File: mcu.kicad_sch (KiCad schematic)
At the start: 34 parts, among them J201 WIFI_ANT, J202 UART, SW201 BOOT_SEL, SW202 RST_SW, U201 ESP32C3, U202 W25Q32JVSS, Y202 40MHz

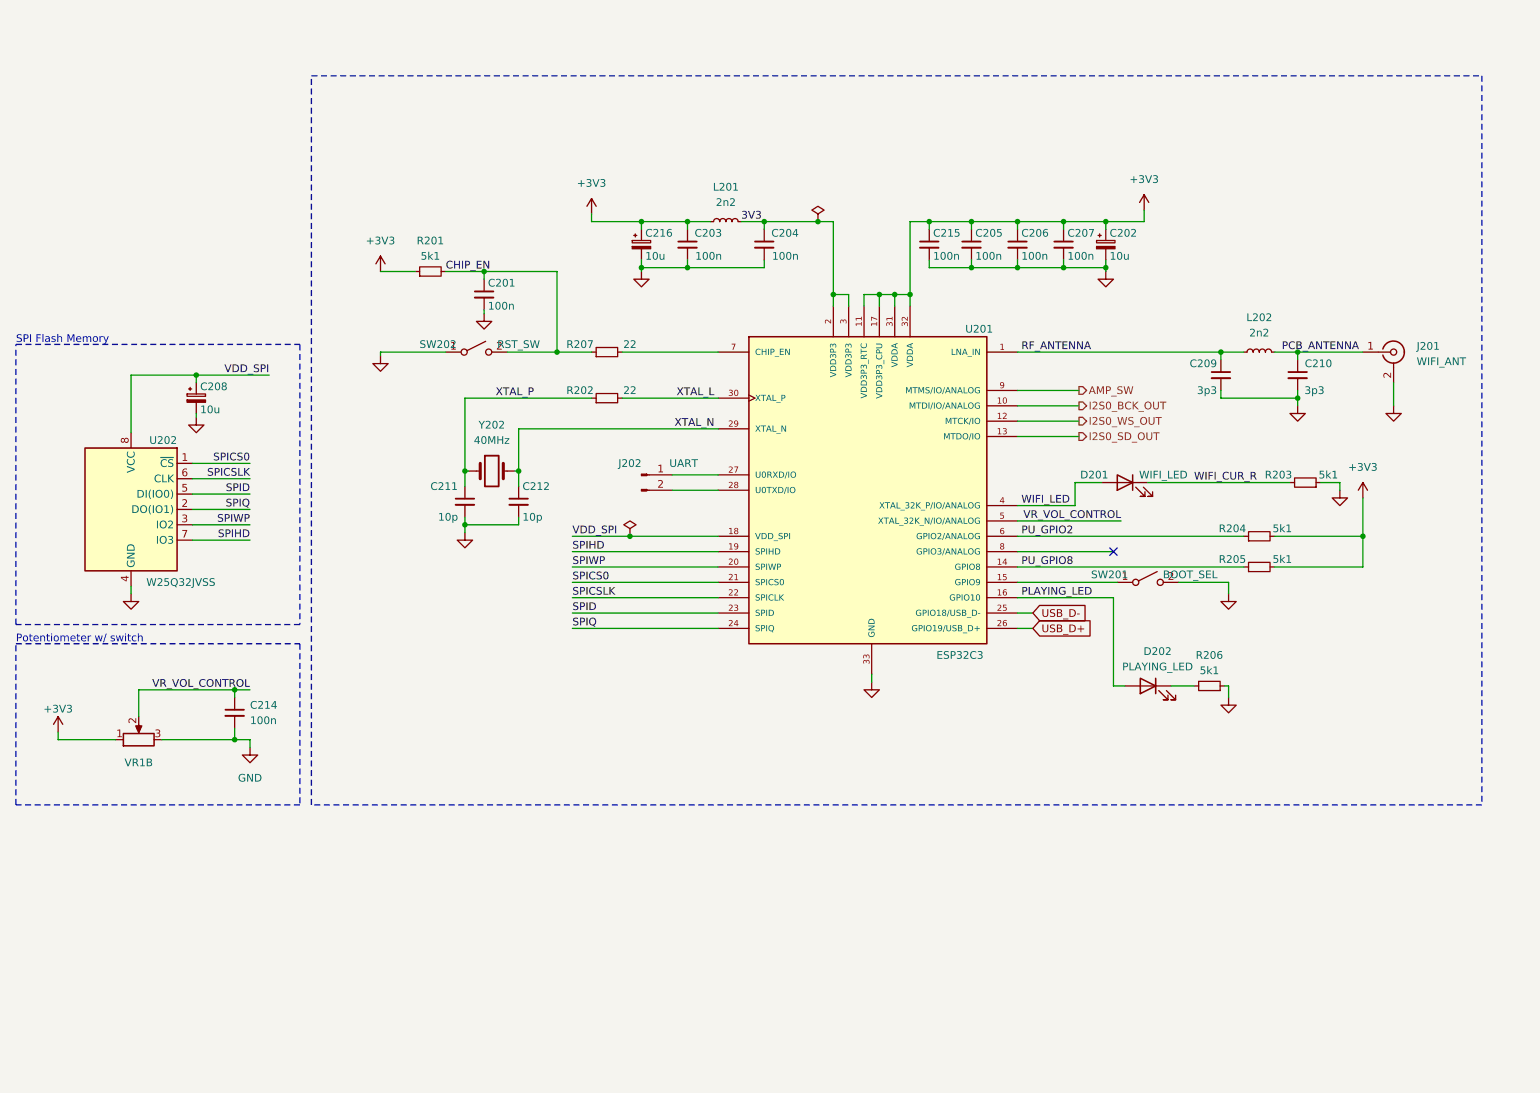
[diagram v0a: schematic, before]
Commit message: updated to rev 4
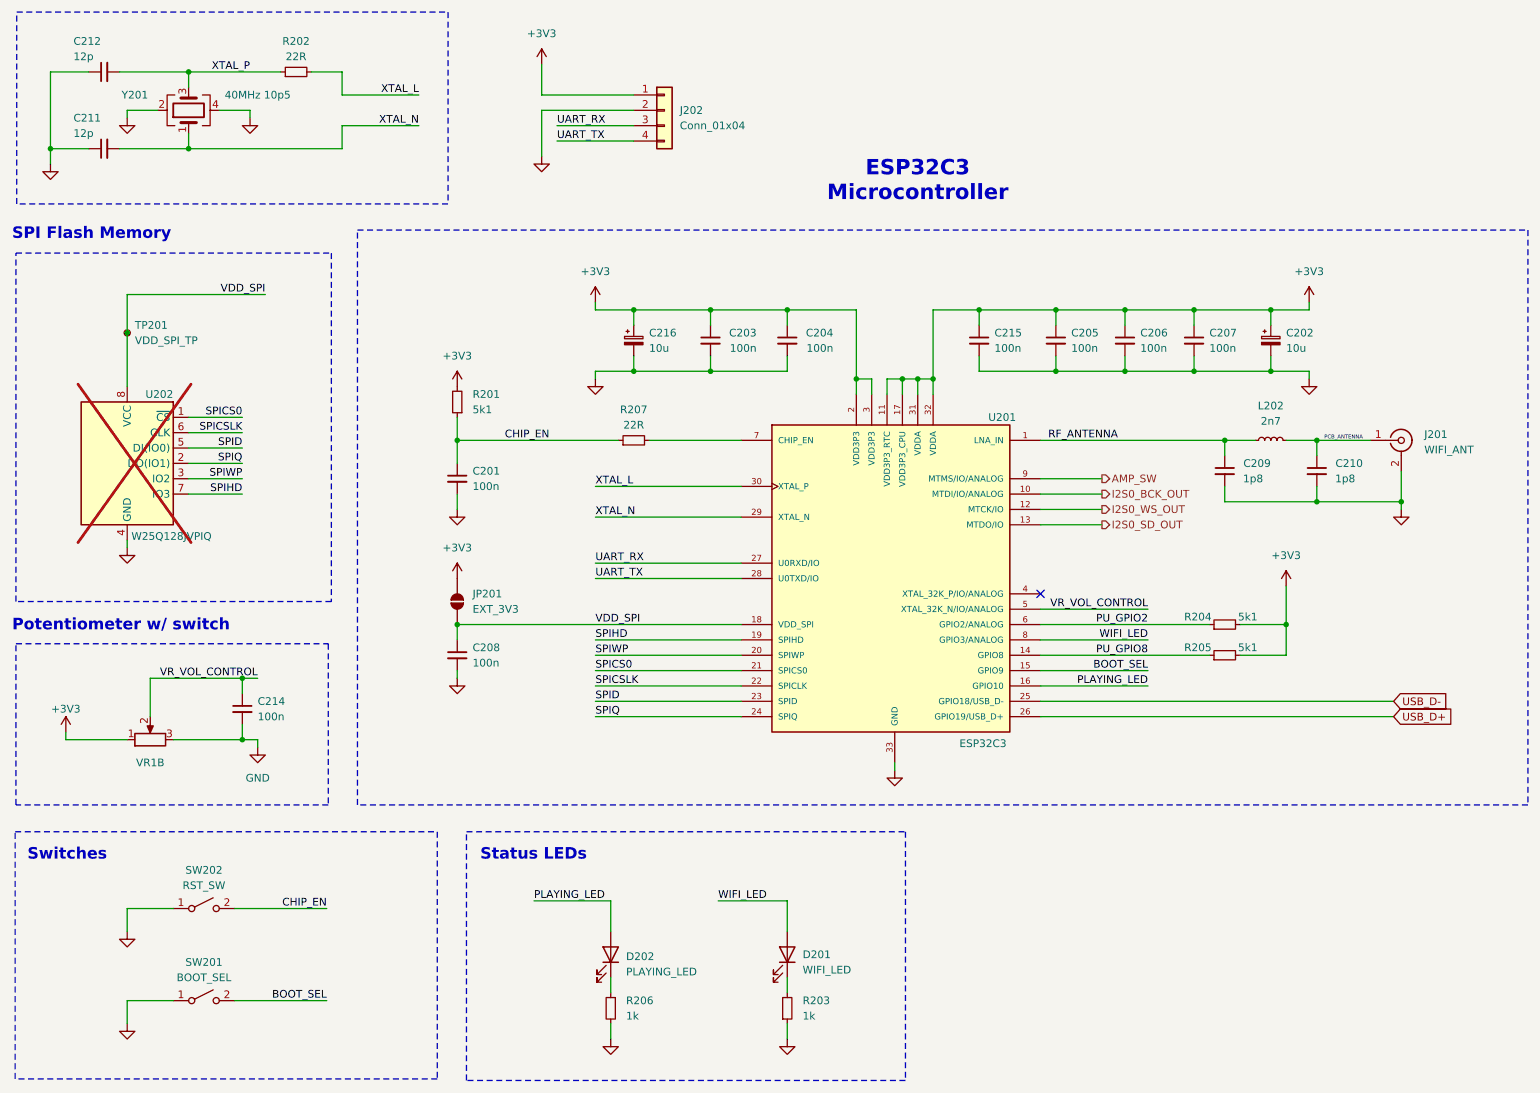
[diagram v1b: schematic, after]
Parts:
- removed C208: 10u, Capacitor_SMD:C_0805_2012Metric, symbol Device:C_Polarized_Small
- removed J202: UART, Connector_PinSocket_2.54mm:PinSocket_1x02_P2.54mm_Vertical, symbol Connector:Conn_01x02_Pin
- removed L201: 2n2, Inductor_SMD:L_0805_2012Metric, symbol Device:L_Small
- removed Y202: 40MHz, Crystal:Crystal_SMD_HC49-SD, symbol Device:Crystal
- added C208: 100n, Capacitor_SMD:C_0402_1005Metric, symbol Device:C_Small
- added J202: Conn_01x04, Connector_PinSocket_2.54mm:PinSocket_1x04_P2.54mm_Vertical, symbol Connector_Generic:Conn_01x04
- added JP201: EXT_3V3, Jumper:SolderJumper-2_P1.3mm_Open_RoundedPad1.0x1.5mm, symbol Jumper:SolderJumper_2_Open
- added TP201: VDD_SPI_TP, TestPoint:TestPoint_Pad_D1.5mm, symbol Connector:TestPoint_Small
- added Y201: 40MHz 10p5, Crystal:Crystal_SMD_3225-4Pin_3.2x2.5mm, symbol Device:Crystal_GND24
- C201, C203, C204, C205, C206, C207, C214, C215: footprint Capacitor_SMD:C_0603_1608Metric -> Capacitor_SMD:C_0402_1005Metric; JLCPCB Part # (none) -> C1525; LCSC C1525 -> (none)
- C202, C216: footprint Capacitor_SMD:C_0805_2012Metric -> Capacitor_SMD:C_0603_1608Metric; JLCPCB Part # (none) -> C96446
- C209, C210: value 3p3 -> 1p8; footprint Capacitor_SMD:C_0603_1608Metric -> Capacitor_SMD:C_0402_1005Metric; JLCPCB Part # (none) -> C1553; LCSC C1565 -> (none)
- C211, C212: value 10p -> 12p; footprint Capacitor_SMD:C_0603_1608Metric -> Capacitor_SMD:C_0402_1005Metric; JLCPCB Part # (none) -> C1547; LCSC C32949 -> (none)
- D201: JLCPCB Part # (none) -> C2297; LCSC C72041 -> (none)
- D202: JLCPCB Part # (none) -> C2296; LCSC C72038 -> (none)
- J201: footprint Connector_Coaxial:SMA_Amphenol_901-143_Horizontal -> Internet_Radio_Speaker:Texas_SWRA117D_2.4GHz_Right
- L202: value 2n2 -> 2n7; footprint Inductor_SMD:L_0805_2012Metric -> Inductor_SMD:L_0402_1005Metric; JLCPCB Part # (none) -> C77108; LCSC C97985 -> (none)
- R201, R204, R205: footprint Resistor_SMD:R_0603_1608Metric -> Resistor_SMD:R_0402_1005Metric; JLCPCB Part # (none) -> C25905; LCSC C25744 -> (none)
- R202, R207: value 22 -> 22R; footprint Resistor_SMD:R_0603_1608Metric -> Resistor_SMD:R_0402_1005Metric; JLCPCB Part # (none) -> C25092; LCSC C25744 -> (none)
- R203, R206: value 5k1 -> 1k; footprint Resistor_SMD:R_0603_1608Metric -> Resistor_SMD:R_0402_1005Metric; JLCPCB Part # (none) -> C11702; LCSC C25905 -> (none)
- SW201, SW202: JLCPCB Part # (none) -> C2889001; LCSC C318884 -> (none)
- U202: value W25Q32JVSS -> W25Q128JVPIQ; footprint Package_SO:SOIC-8_3.9x4.9mm_P1.27mm -> Package_SON:WSON-8-1EP_6x5mm_P1.27mm_EP3.4x4.3mm; JLCPCB Part # (none) -> C190862; LCSC C179173 -> (none); now not fitted; now left out of the parts list
- VR1: JLCPCB Part # (none) -> C2687318; LCSC C2687318 -> (none)
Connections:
- net 3V3 is gone; now on net +3V3: C204.1, U201.2 (VDD3P3), U201.3 (VDD3P3)
- net +3V3: now also R201.2, J202.1 (Pin_1), JP201.2 (B); no longer R201.1
- net CHIP_EN: now also R201.1; no longer R201.2
- net GND: now also C211.1, C212.1, R206.2, SW201.1 (A), C208.2, J202.2 (Pin_2), Y201.2, Y201.4; no longer C211.2, C212.2, R206.1, SW201.2 (B)
- net VDD_SPI: now also C208.1, JP201.1 (A), TP201.1
- net WIFI_LED: now also U201.8 (GPIO3/ANALOG); no longer U201.4 (XTAL_32K_P/IO/ANALOG)
- net XTAL_N: now also C211.2, Y201.1; no longer C212.1
- net XTAL_P: now also C212.2, Y201.3; no longer C211.1
- net at D202.1 (K): now also R206.1; no longer R206.2
- net BOOT_SEL: now reaches U201.15 (GPIO9)
- net BOOT_SEL: now also SW201.2 (B); no longer SW201.1 (A)
- net UART_RX: now reaches U201.27 (U0RXD/IO)
- net UART_RX: now also J202.3 (Pin_3)
- net UART_TX: now reaches U201.28 (U0TXD/IO)
- net UART_TX: now also J202.4 (Pin_4)
- net WIFI_CUR_R: no longer names the net of D201.1 (K), R203.2
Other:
- note added: "ESP32C3 Microcontroller"
- note added: "Status LEDs"
- note added: "Switches"
- moved on the sheet: C201, C202, C203, C204, C205, C206, C207, C209, C210, C211, C212, C214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
